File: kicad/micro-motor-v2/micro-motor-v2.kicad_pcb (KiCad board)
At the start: 2 copper layers, 35 x 20 mm, 78 parts, among them J101 SUPPLY, J102 SW, J103 Hall, J104 Encoder, J105 NTC, J106 Motor, J201 CAN, J301 USB, J302 UART, J303 SWD, Q401 FDMD82xx, Q402 FDMD82xx, Q403 FDMD82xx, U201 TCAN332, U301 STM32G474CET6, U401 DRV8320S, U402 INA240A2PW, U403 INA240A2PW, U404 INA240A2PW, U501 TPS82150, U502 TPS82150

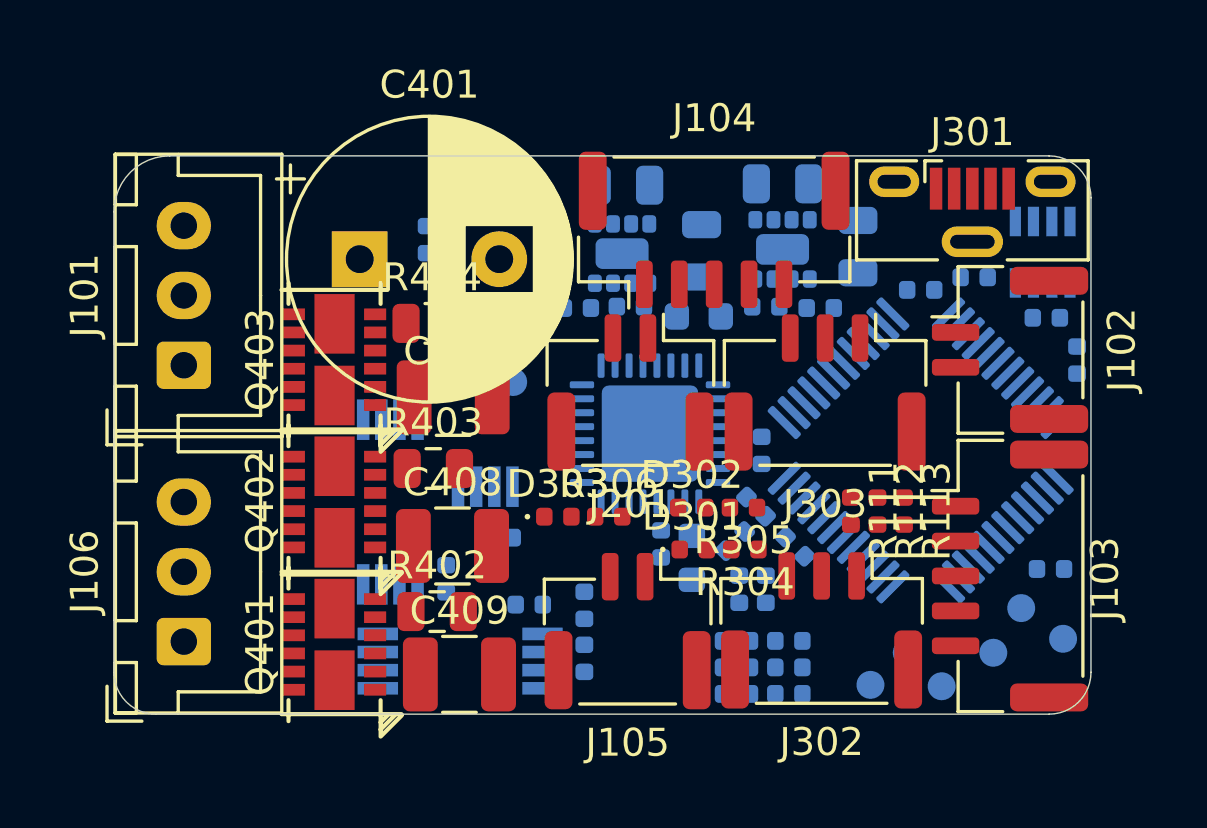
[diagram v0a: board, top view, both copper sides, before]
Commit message: micro-motor-v2: Layout...
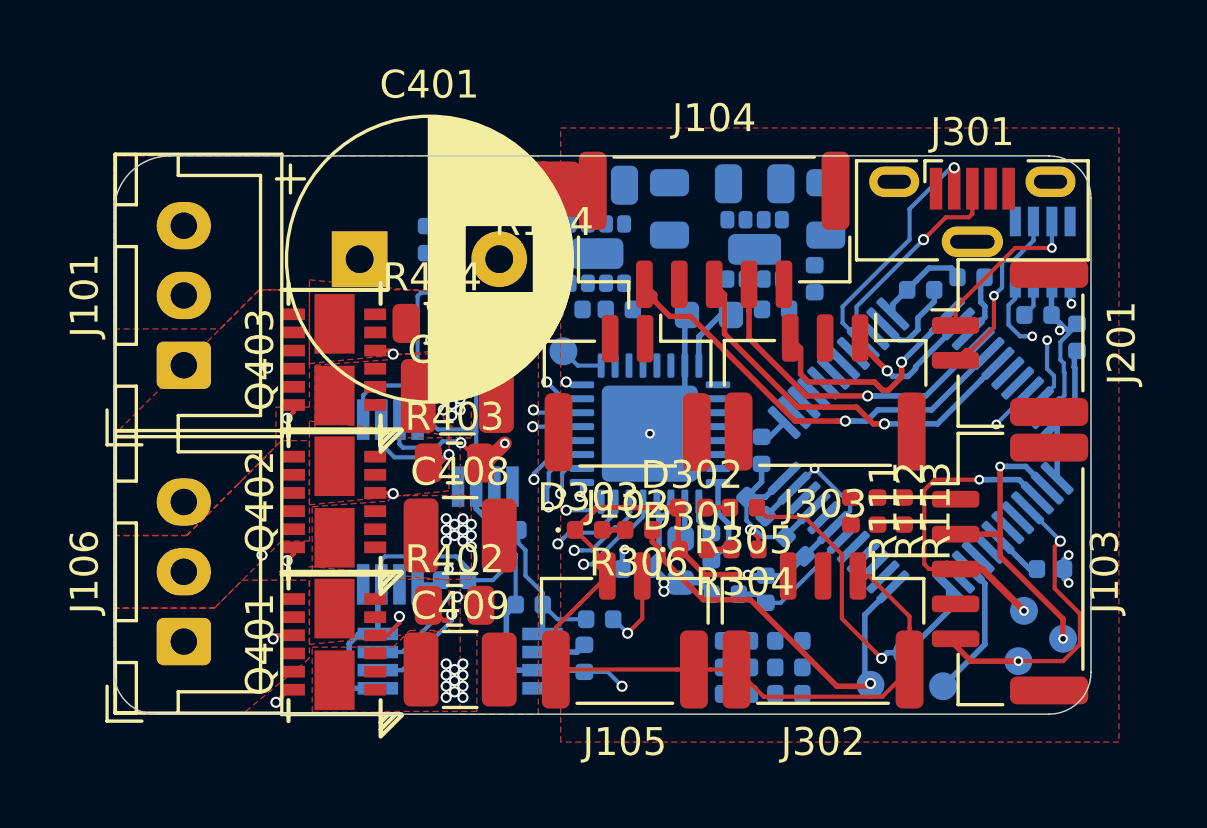
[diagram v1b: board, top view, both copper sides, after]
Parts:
- added R114: 0, Resistor_SMD:R_0402_1005Metric, F.Cu at (165.4, 101.2)
- moved J102 13.8 mm to (168.4, 108.5), turned to 180 degrees
- moved J201 13.7 mm to (182.1, 106.7), turned to 270 degrees
- moved TP303 3.96 mm to (179.7, 119.0)
- moved TP103 2.89 mm to (182.4, 118.1)
- moved TP401 2.11 mm to (166.1, 107.0)
- moved C504 1.89 mm to (169.9, 101.9)
- moved TP102 1.86 mm to (182.6, 116.3)
- moved C503 1.77 mm to (175.5, 101.9)
- moved C402 1.27 mm to (168.7, 114.8), turned to 180 degrees
- moved D303 1.20 mm to (167.0, 113.4)
- moved R306 1.18 mm to (168.8, 113.4), turned to 180 degrees
- moved R501 1.07 mm to (175.1, 104.4), turned to 270 degrees
- moved C502 1.00 mm to (172.9, 101.0)
- moved U501 1.00 mm to (172.9, 103.3)
- moved C501 0.90 mm to (167.3, 101.0)
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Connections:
- net Net-(J201-Pad1) renamed /Can/CANH
- net Net-(J201-Pad2) renamed /Can/CANL
- net Net-(Q401-Pad14) renamed /Motordriver/GND_A
- net Net-(Q402-Pad14) renamed /Motordriver/GND_B
- net Net-(Q403-Pad14) renamed /Motordriver/GND_C
- C401 pad 2: GND -> GNDPWR
- C402 pad 2: GND -> GNDPWR
- C403 pad 2: GND -> GNDPWR
- C404 pad 2: GND -> GNDPWR
- C407 pad 2: GND -> GNDPWR
- C408 pad 2: GND -> GNDPWR
- C409 pad 2: GND -> GNDPWR
- J101 pad 2: GND -> GNDPWR
- R402 pad 2: GND -> GNDPWR
- R403 pad 2: GND -> GNDPWR
- R404 pad 2: GND -> GNDPWR
- U301 pad 17: /Microcontroller/ADC_Vsupply -> /Microcontroller/ADC_NTC
- U301 pad 18: /Microcontroller/ADC_NTC -> /Microcontroller/ADC_Vsupply
- U401 pad 23: GND -> GNDPWR
- U401 pad 31: GND -> GNDPWR
- U401 pad 33: GND -> GNDPWR
- U402 pad 3: GND -> GNDPWR
- U403 pad 3: GND -> GNDPWR
- U404 pad 3: GND -> GNDPWR
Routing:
- net GND: track 0.00 -> 94.3 mm, vias 0 -> 6
- net GNDPWR: track 0.00 -> 32.9 mm, vias 0 -> 6
- net +3V3: track 0.00 -> 26.3 mm, vias 0 -> 2
- net Net-(Q401-Pad12): track 0.00 -> 17.3 mm, vias 0 -> 2
- net /Motordriver/OUT_U: track 0.00 -> 15.9 mm, vias 0 -> 2
- net +24V: track 0.00 -> 15.6 mm, vias 0 -> 35
- net /Microcontroller/B: track 0.00 -> 15.5 mm, vias 0 -> 1
- net /Microcontroller/DAC2: track 0.00 -> 14.5 mm, vias 0 -> 1
- net /Motordriver/OUT_V: track 0.00 -> 14.3 mm, vias 0 -> 2
- net /Microcontroller/A: track 0.00 -> 14.0 mm, vias 0 -> 1
- net Net-(Q402-Pad12): track 0.00 -> 13.0 mm, vias 0 -> 2
- net /Motordriver/OUT_W: track 0.00 -> 12.1 mm, vias 0 -> 2
- net /Microcontroller/DAC1: track 0.00 -> 12.0 mm, vias 0 -> 1
- net /Motordriver/GND_A: track 0.00 -> 11.8 mm, vias 0 -> 2
- net /Microcontroller/INDEX: track 0.00 -> 11.8 mm, vias 0 -> 1
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- added copper zone on F.Cu, net +24V
- added copper zone on In1.Cu, net +24V
- added copper zone on F.Cu, net /Motordriver/GND_A
- added copper zone on F.Cu, net /Motordriver/GND_B
- added copper zone on F.Cu, net /Motordriver/GND_C
- added copper zone on F.Cu, net /Motordriver/OUT_U
- added copper zone on F.Cu, net /Motordriver/OUT_V
- added copper zone on F.Cu, net /Motordriver/OUT_W
- added copper zone on F.Cu, net GND
- added copper zone on In1.Cu, net GND
- added copper zone on F.Cu, net GNDPWR
- added copper zone on In1.Cu, net GNDPWR
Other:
- copper layers 2 -> 4
- rule pad_to_mask_clearance: 0.051 -> 0.025
- rule solder_mask_min_width: 0.25 -> 0.1
- rule trace_min: 0.2 -> 0.125
- rule via_min_drill: 0.3 -> 0.2
- rule via_min_size: 0.4 -> 0.3

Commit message: micro-motor-v2: Layout...
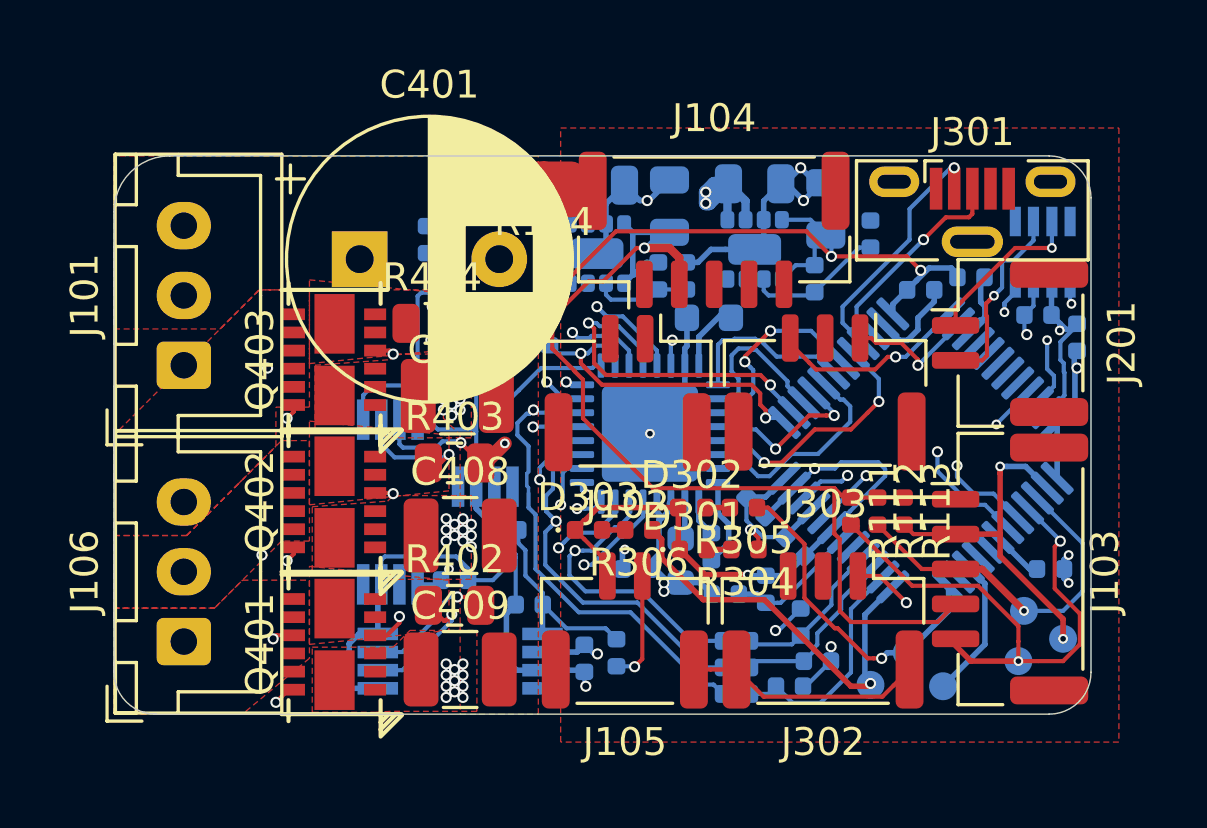
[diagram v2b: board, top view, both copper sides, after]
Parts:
- moved R401 8.71 mm to (165.6, 106.3), turned to 270 degrees
- moved R504 4.37 mm to (170.5, 104.3), turned to 90 degrees
- moved R502 4.34 mm to (177.1, 102.8), turned to 90 degrees
- moved TP401 2.89 mm to (163.8, 108.8)
- moved R503 1.84 mm to (169.5, 104.3), turned to 270 degrees
- moved R108 1.34 mm to (168.0, 117.8), turned to 270 degrees
- moved R105 1.05 mm to (175.2, 118.1)
- moved R103 0.80 mm to (174.6, 116.7), turned to 90 degrees
- moved R107 0.28 mm to (174.2, 119.0)
- moved C504 0.10 mm to (169.9, 101.8)
- moved C404 0.10 mm to (171.3, 105.8)
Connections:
- R102 pad 1: /Motordriver/OUT_W -> /Motordriver/OUT_U
- R102 pad 2: /Microcontroller/Volt_W -> /Microcontroller/Volt_U
- R103 pad 1: /Microcontroller/Volt_W -> /Microcontroller/Volt_U
- R106 pad 1: /Motordriver/OUT_U -> /Motordriver/OUT_W
- R106 pad 2: /Microcontroller/Volt_U -> /Microcontroller/Volt_W
- R107 pad 1: /Microcontroller/Volt_U -> /Microcontroller/Volt_W
- U301 pad 14: /Microcontroller/Volt_U -> /Microcontroller/Volt_W
- U301 pad 16: /Microcontroller/Volt_W -> /Microcontroller/Volt_U
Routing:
- net +3V3: track 26.3 -> 71.6 mm, vias 2 -> 7
- net +5V: track 0.00 -> 38.9 mm, vias 0 -> 1
- net +6V: track 0.00 -> 32.4 mm, vias 0 -> 4
- net /Microcontroller/~CS: track 0.00 -> 22.7 mm, vias 0 -> 2
- net /Microcontroller/ENABLE: track 0.00 -> 18.3 mm, vias 0 -> 2
- net /Motordriver/MOSI: track 0.00 -> 17.3 mm, vias 0 -> 2
- net /Microcontroller/VREF: track 1.61 -> 17.2 mm, vias 0 -> 2
- net /Microcontroller/B: track 15.5 -> 0.00 mm, vias 1 -> 0
- net /Motordriver/OUT_W: track 12.1 -> 27.0 mm
- net /Microcontroller/A: track 14.0 -> 0.00 mm, vias 1 -> 0
- net /Motordriver/SCK: track 0.00 -> 12.4 mm, vias 0 -> 2
- net /Microcontroller/INDEX: track 11.8 -> 0.00 mm, vias 1 -> 0
- net /Motordriver/MISO: track 1.02 -> 12.1 mm, vias 0 -> 2
- net /Motordriver/OUT_V: track 14.3 -> 25.1 mm
- net /Motordriver/IN_W_P: track 0.00 -> 9.10 mm, vias 0 -> 2
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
